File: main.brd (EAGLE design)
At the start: 65.7 x 40.6 mm, 18 parts, among them IC1 ATMEGA328P-PU, IC2 LM7805, J1 2,1mm, Q1 16 MHz

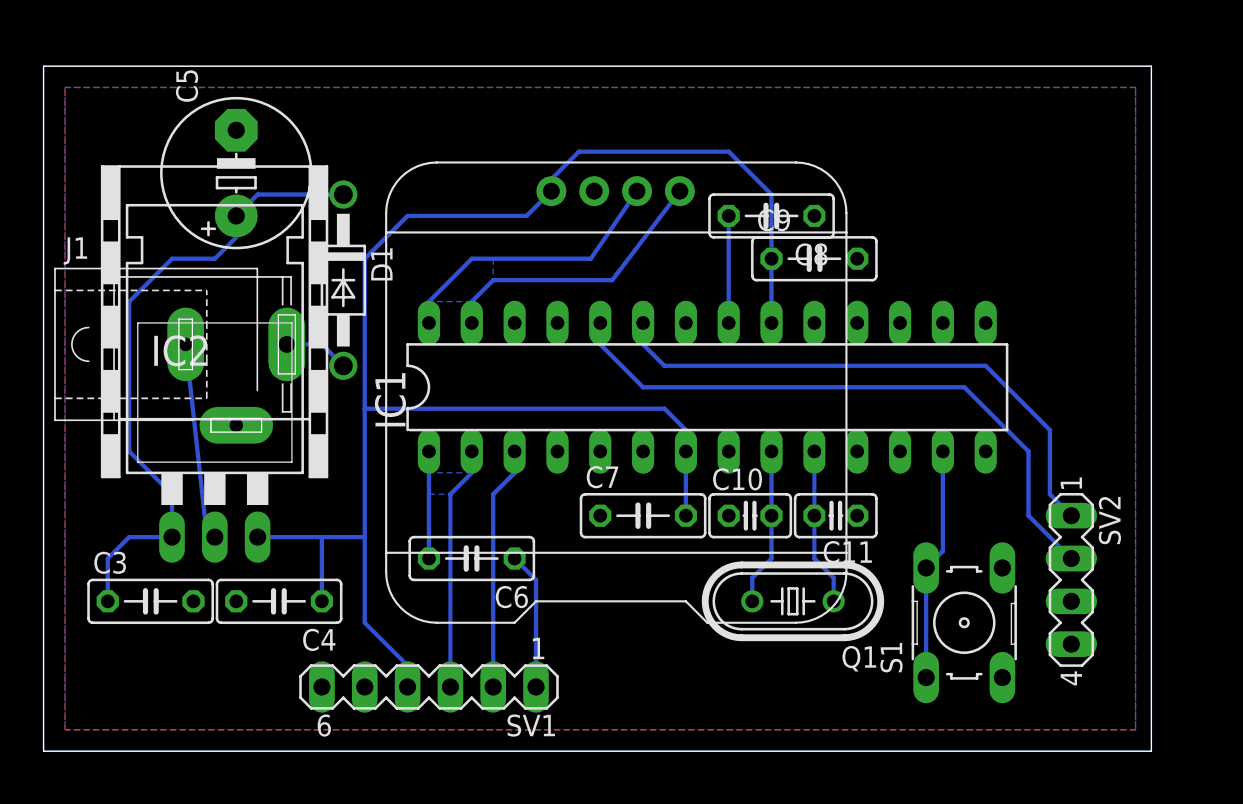
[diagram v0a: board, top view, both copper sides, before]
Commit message: Opravy
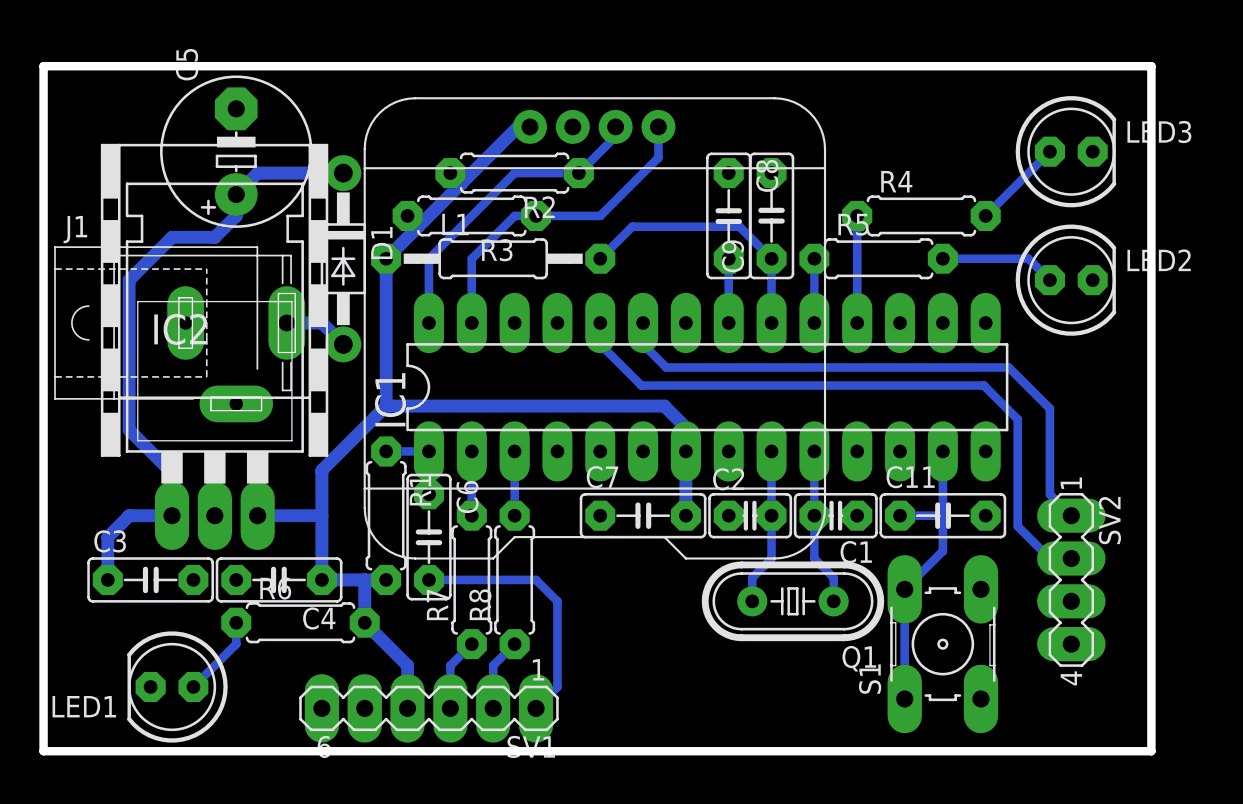
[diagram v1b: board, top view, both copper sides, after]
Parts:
- added C1: 22 pF, rcl:C025-025X050
- added L1: EC24-100K, rcl:0207/12
- added LED1: Red, led:LED5MM
- added LED2: Green, led:LED5MM
- added LED3: Yellow, led:LED5MM
- added R1, R4, R5, R6, R7, R8: (no value), rcl:0207/7
- added R2, R3: 10K, rcl:0207/7
- C11: value 22 pF -> 0,1 μF; device rcl:C025-025X050 -> rcl:C050-025X075
- S1: value (none) -> TC-0103-T
- moved C11 6.35 mm to (53.3, 14.0), turned to 0 degrees
- moved U$1 4.02 mm to (33.0, 25.4)
- moved C9 3.59 mm to (43.2, 31.8), turned to 90 degrees
- moved C6 2.84 mm to (22.9, 12.7), turned to 270 degrees
- moved C8 2.54 mm to (40.6, 31.8), turned to 270 degrees
- moved S1 1.80 mm to (53.3, 6.35)
- moved C5 1.27 mm to (11.4, 35.6)
- moved SV1 1.27 mm to (22.9, 2.54)
- moved C3 1.27 mm to (6.35, 10.2)
- moved C4 1.27 mm to (14.0, 10.2)
- moved D1 1.27 mm to (17.8, 29.2)
- moved IC2 1.27 mm to (10.2, 19.1)
- moved J1 1.27 mm to (11.4, 25.4)
- renumbered C10 to C2
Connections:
- new net N$14: IC1.18, R4.1
- new net N$16: IC1.19, R5.1
- new net N$17: LED3.A, R4.2
- new net N$18: C9.1, IC1.20, L1.2
- new net N$19: LED2.A, R5.2
- new net N$20: LED1.A, R6.1
- new net N$21: R8.1, SV1.2
- new net N$22: R7.1, SV1.3
- net +5V: now also L1.1, R1.2, R2.2, R3.2, R6.2; no longer C9.1, IC1.20
- net GND: now also C1.1, C11.2, LED1.K, LED2.K, LED3.K; no longer C11.1
- net N$1: now also C1.2; no longer C11.2
- net N$3: now also R3.1
- net N$4: now also R2.1
- net N$5: now also C6.1, R1.1; no longer C6.2
- net N$6: now also C11.1
- net N$7: now also C6.2; no longer C6.1
- net N$8: now also R7.2; no longer SV1.3
- net N$9: now also R8.2; no longer SV1.2
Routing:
- net N$16: track 172.1 -> 3.81 mm
- net N$17: track 40.6 -> 5.39 mm
- net +5V: track 97.1 -> 75.7 mm
- net N$18: track 0.00 -> 15.5 mm
- net GND: track 11.5 -> 0.00 mm
- net N$9: track 14.5 -> 3.81 mm
- net N$8: track 14.5 -> 5.08 mm
- net N$7: track 8.15 -> 15.0 mm
- net N$19: track 0.00 -> 6.88 mm
- net N$14: track 0.00 -> 6.35 mm
- net N$20: track 0.00 -> 4.86 mm
- net N$6: track 13.8 -> 18.2 mm
- net N$22: track 0.00 -> 4.34 mm
- net N$21: track 0.00 -> 4.34 mm
- net N$12: track 6.35 -> 3.81 mm
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- added copper zone on layer 1, net GND
- removed copper zone on layer 16, net LL
- removed copper zone on layer 16, net N$14
- removed copper zone on layer 1, net N$15

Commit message: Revize 0.0.1
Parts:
- R1: value (none) -> 10K
- R4, R5, R6: value (none) -> 330
- R7, R8: value (none) -> 1K
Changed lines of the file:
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@@
 <element name="C1" library="rcl" library_urn="urn:adsk.eagle:library:334" package="C025-025X050" value="22 pF" x="46.99" y="13.97" rot="R180"/>
 <element name="L1" library="rcl" library_urn="urn:adsk.eagle:library:334" package="0207/12" value="EC24-100K" x="26.67" y="29.21"/>
-<element name="R1" library="rcl" library_urn="urn:adsk.eagle:library:334" package="0207/7" value="" x="20.32" y="13.97" rot="R270"/>
+<element name="R1" library="rcl" library_urn="urn:adsk.eagle:library:334" package="0207/7" value="10K" x="20.32" y="13.97" rot="R270"/>
 <element name="R2" library="rcl" library_urn="urn:adsk.eagle:library:334" package="0207/7" value="10K" x="27.94" y="34.29" rot="R180"/>
 <element name="R3" library="rcl" library_urn="urn:adsk.eagle:library:334" package="0207/7" value="10K" x="25.4" y="31.75" rot="R180"/>
@@
 <element name="LED2" library="led" library_urn="urn:adsk.eagle:library:259" package="LED5MM" value="Green" x="60.96" y="27.94"/>
 <element name="LED3" library="led" library_urn="urn:adsk.eagle:library:259" package="LED5MM" value="Yellow" x="60.96" y="35.56"/>
-<element name="R4" library="rcl" library_urn="urn:adsk.eagle:library:334" package="0207/7" value="" x="52.07" y="31.75"/>
-<element name="R5" library="rcl" library_urn="urn:adsk.eagle:library:334" package="0207/7" value="" x="49.53" y="29.21"/>
-<element name="R6" library="rcl" library_urn="urn:adsk.eagle:library:334" package="0207/7" value="" x="15.24" y="7.62"/>
-<element name="R7" library="rcl" library_urn="urn:adsk.eagle:library:334" package="0207/7" value="" x="25.4" y="10.16" rot="R90"/>
-<element name="R8" library="rcl" library_urn="urn:adsk.eagle:library:334" package="0207/7" value="" x="27.94" y="10.16" rot="R90"/>
+<element name="R4" library="rcl" library_urn="urn:adsk.eagle:library:334" package="0207/7" value="330" x="52.07" y="31.75"/>
+<element name="R5" library="rcl" library_urn="urn:adsk.eagle:library:334" package="0207/7" value="330" x="49.53" y="29.21"/>
+<element name="R6" library="rcl" library_urn="urn:adsk.eagle:library:334" package="0207/7" value="330" x="15.24" y="7.62"/>
+<element name="R7" library="rcl" library_urn="urn:adsk.eagle:library:334" package="0207/7" value="1K" x="25.4" y="10.16" rot="R90"/>
+<element name="R8" library="rcl" library_urn="urn:adsk.eagle:library:334" package="0207/7" value="1K" x="27.94" y="10.16" rot="R90"/>
 </elements>
 <signals>

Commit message: Opravy na celorepublikové kolo
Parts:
- OLED: value OLED_0.96_I2C -> 128x64 SSD1306 I2C
- renumbered U$1 to OLED
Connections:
- net N$13 renamed IJVCC
- net N$4 renamed SCL
- net N$6 renamed BTN
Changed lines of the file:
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@@
 <?xml version="1.0" encoding="utf-8"?>
 <!DOCTYPE eagle SYSTEM "eagle.dtd">
-<eagle version="8.2.0">
+<eagle version="8.2.1">
 <drawing>
 <settings>
@@
 <layer number="17" name="Pads" color="2" fill="1" visible="yes" active="yes"/>
 <layer number="18" name="Vias" color="2" fill="1" visible="yes" active="yes"/>
-<layer number="19" name="Unrouted" color="6" fill="1" visible="yes" active="yes"/>
+<layer number="19" name="Unrouted" color="6" fill="1" visible="no" active="yes"/>
 <layer number="20" name="Dimension" color="15" fill="1" visible="yes" active="yes"/>
-<layer number="21" name="tPlace" color="7" fill="1" visible="yes" active="yes"/>
-<layer number="22" name="bPlace" color="7" fill="1" visible="yes" active="yes"/>
-<layer number="23" name="tOrigins" color="15" fill="1" visible="yes" active="yes"/>
-<layer number="24" name="bOrigins" color="15" fill="1" visible="yes" active="yes"/>
+<layer number="21" name="tPlace" color="7" fill="1" visible="no" active="yes"/>
+<layer number="22" name="bPlace" color="7" fill="1" visible="no" active="yes"/>
+<layer number="23" name="tOrigins" color="15" fill="1" visible="no" active="yes"/>
+<layer number="24" name="bOrigins" color="15" fill="1" visible="no" active="yes"/>
 <layer number="25" name="tNames" color="7" fill="1" visible="no" active="yes"/>
 <layer number="26" name="bNames" color="7" fill="1" visible="no" active="yes"/>
@@
 <layer number="49" name="Reference" color="7" fill="1" visible="no" active="yes"/>
 <layer number="50" name="dxf" color="7" fill="1" visible="no" active="no"/>
-<layer number="51" name="tDocu" color="7" fill="1" visible="yes" active="yes"/>
-<layer number="52" name="bDocu" color="7" fill="1" visible="yes" active="yes"/>
+<layer number="51" name="tDocu" color="7" fill="1" visible="no" active="yes"/>
+<layer number="52" name="bDocu" color="7" fill="1" visible="no" active="yes"/>
 <layer number="53" name="tGND_GNDA" color="7" fill="9" visible="no" active="no"/>
 <layer number="54" name="bGND_GNDA" color="1" fill="9" visible="no" active="no"/>
@@
 <attribute name="OC_NEWARK" value="unknown" x="22.86" y="2.54" size="1.778" layer="27" rot="R180" display="off"/>
 </element>
-<element name="U$1" library="tft_1.8_1.44_oled_0.96" package="OLED_0.96_I2C" value="OLED_0.96_I2C" x="33.02" y="25.4"/>
+<element name="OLED" library="tft_1.8_1.44_oled_0.96" package="OLED_0.96_I2C" value="128x64 SSD1306 I2C" x="33.02" y="25.4"/>
 <element name="IC2" library="78xx_with_heatsink" package="78XXH" value="LM7805" x="10.16" y="19.05"/>
 <element name="S1" library="switch-omron" library_urn="urn:adsk.eagle:library:377" package="B3F-10XX" value="TC-0103-T" x="53.34" y="6.35" rot="R90">
@@
 <contactref element="C5" pad="-"/>
 <contactref element="SV1" pad="6"/>
-<contactref element="U$1" pad="GND"/>
+<contactref element="OLED" pad="GND"/>
 <polygon width="0.762" layer="16" isolate="0.762" thermals="no">
 <vertex x="0" y="0"/>
@@
 <contactref element="C4" pad="1"/>
 <contactref element="SV1" pad="4"/>
-<contactref element="U$1" pad="VCC"/>
+<contactref element="OLED" pad="VCC"/>
 <contactref element="IC2" pad="OUT"/>
 <wire x1="19.05" y1="10.16" x2="19.05" y2="7.62" width="0.762" layer="16"/>
@@
 <signal name="N$3">
 <contactref element="IC1" pad="27"/>
-<contactref element="U$1" pad="SDA"/>
+<contactref element="OLED" pad="SDA"/>
 <wire x1="25.4" y1="25.4" x2="25.4" y2="29.21" width="0.508" layer="16"/>
 <wire x1="27.94" y1="31.75" x2="25.4" y2="29.21" width="0.508" layer="16"/>
@@
 <wire x1="29.21" y1="31.75" x2="33.02" y2="31.75" width="0.508" layer="16"/>
 </signal>
-<signal name="N$4">
+<signal name="SCL">
 <contactref element="IC1" pad="28"/>
 <wire x1="22.86" y1="25.4" x2="22.86" y2="29.21" width="0.508" layer="16"/>
 <wire x1="22.86" y1="29.21" x2="27.94" y2="34.29" width="0.508" layer="16"/>
-<contactref element="U$1" pad="SCL"/>
+<contactref element="OLED" pad="SCL"/>
 <contactref element="R2" pad="1"/>
 <wire x1="27.94" y1="34.29" x2="31.75" y2="34.29" width="0.508" layer="16"/>
@@
 <wire x1="27.94" y1="17.78" x2="27.94" y2="13.97" width="0.508" layer="16"/>
 </signal>
-<signal name="N$6">
+<signal name="BTN">
 <contactref element="IC1" pad="13"/>
 <contactref element="S1" pad="1"/>
@@
 <wire x1="40.64" y1="29.21" x2="40.64" y2="25.4" width="0.508" layer="16"/>
 </signal>
-<signal name="N$13">
+<signal name="IJVCC">
 <contactref element="J1" pad="3"/>
 <contactref element="D1" pad="A"/>
